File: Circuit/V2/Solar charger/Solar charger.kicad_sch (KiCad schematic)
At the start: 1 part

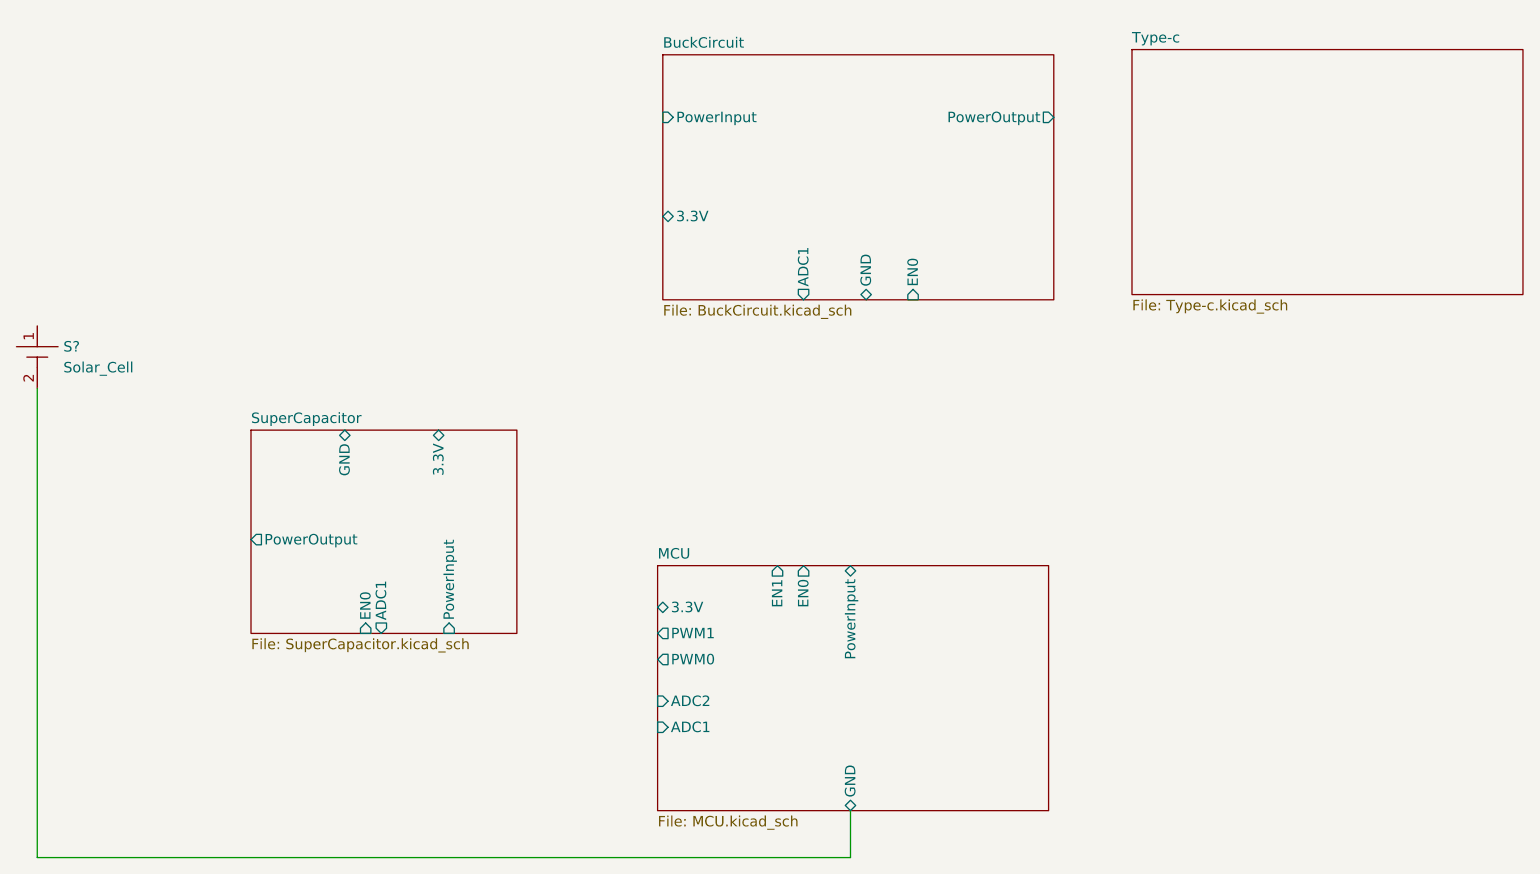
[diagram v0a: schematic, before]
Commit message: update
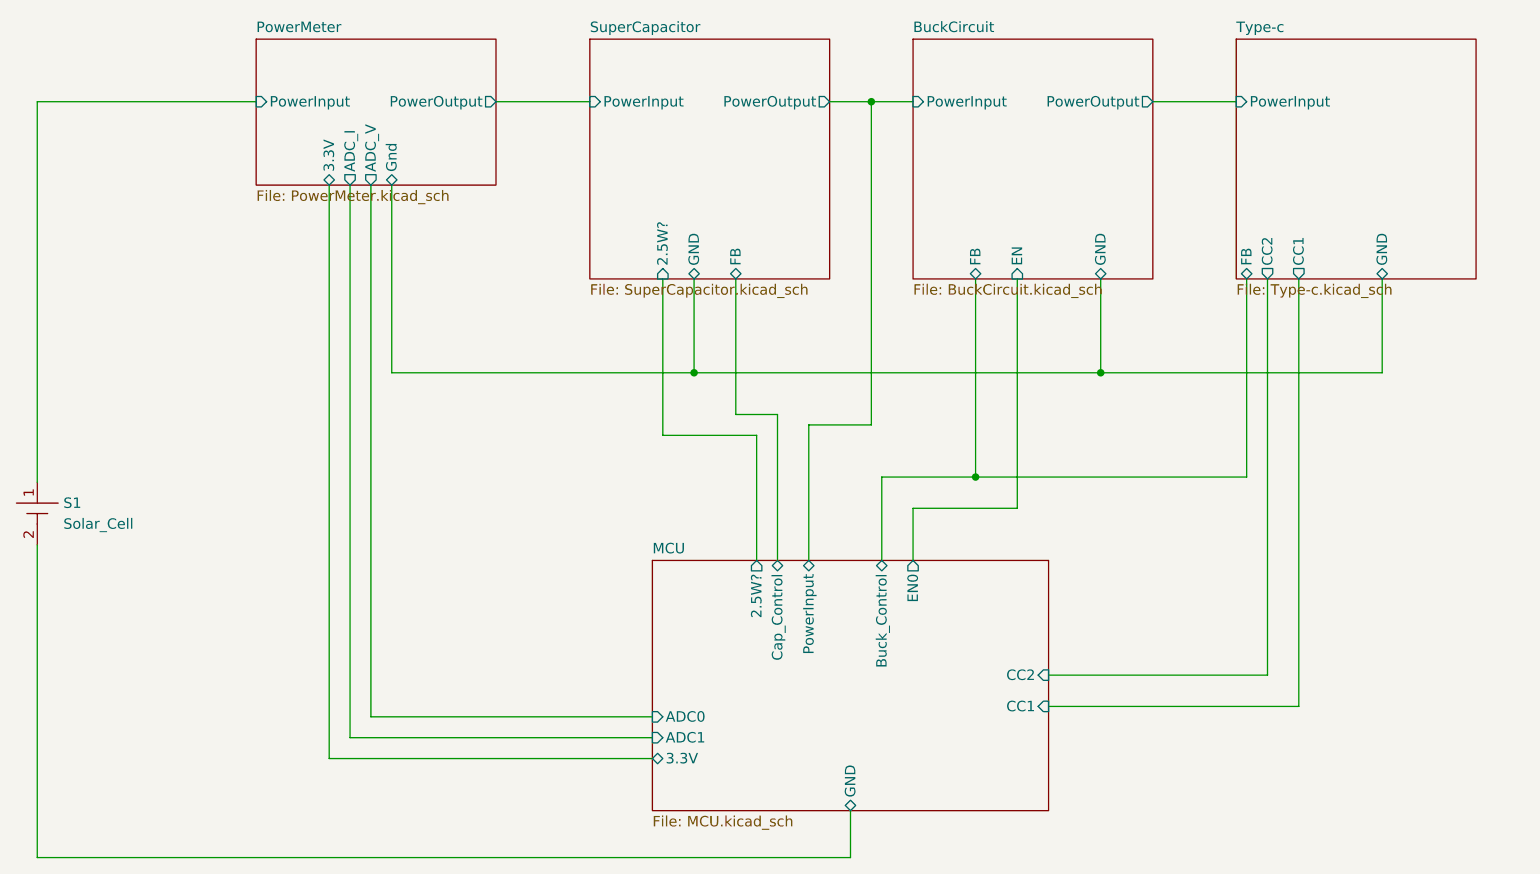
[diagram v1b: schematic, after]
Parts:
- gave numbers to parts that had none: 1
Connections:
- net PowerMeter/PowerInput: now reaches S1.1
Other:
- added sheet PowerMeter (PowerMeter.kicad_sch)
- sheet BuckCircuit ports: added EN, FB; removed 3.3V, ADC1, EN0
- sheet MCU ports: added 2.5W?, ADC0, Buck_Control, CC1, CC2, Cap_Control; removed ADC2, EN1, PWM0, PWM1
- sheet SuperCapacitor ports: added 2.5W?, FB; removed 3.3V, ADC1, EN0
- sheet Type-c ports: added CC1, CC2, FB, GND, PowerInput; removed none
- moved on the sheet: S1
